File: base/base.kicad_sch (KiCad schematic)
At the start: 1 part, among them U1 ESP32-WROOM-32

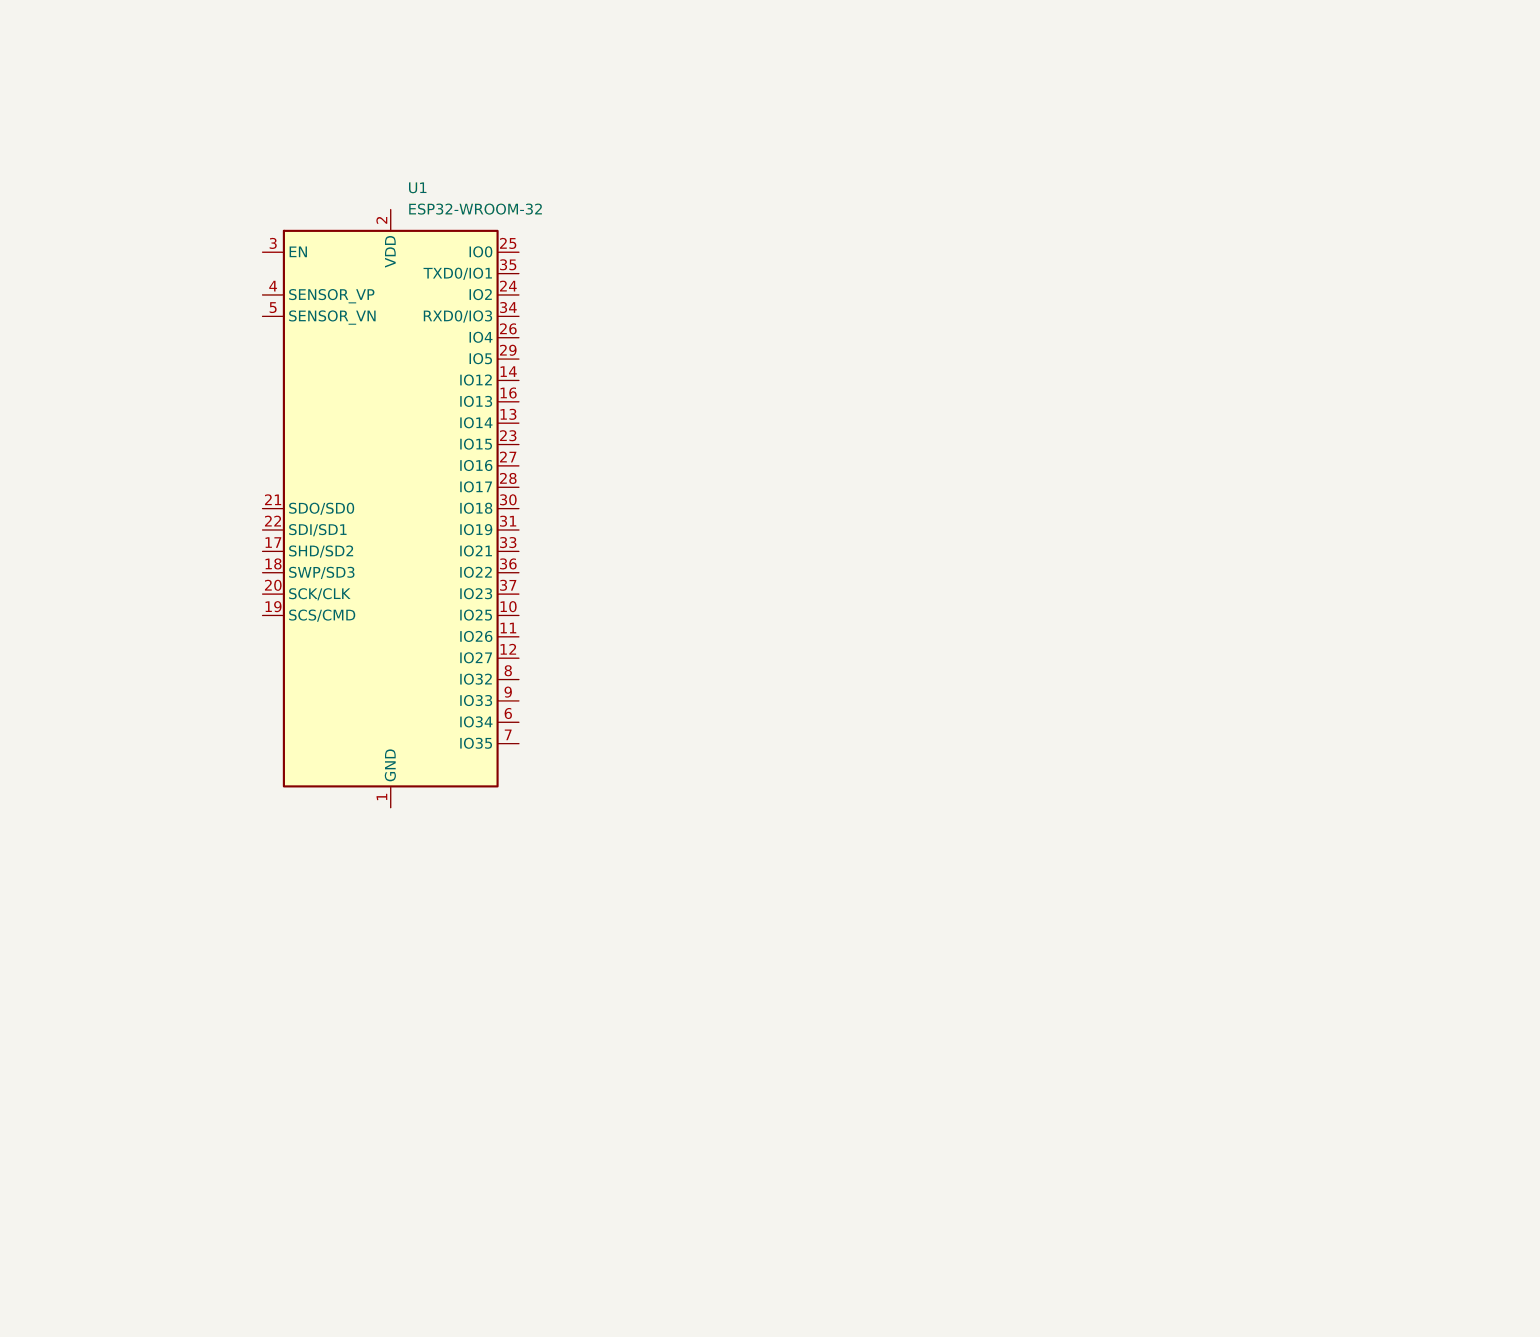
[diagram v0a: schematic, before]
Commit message: add base pcb
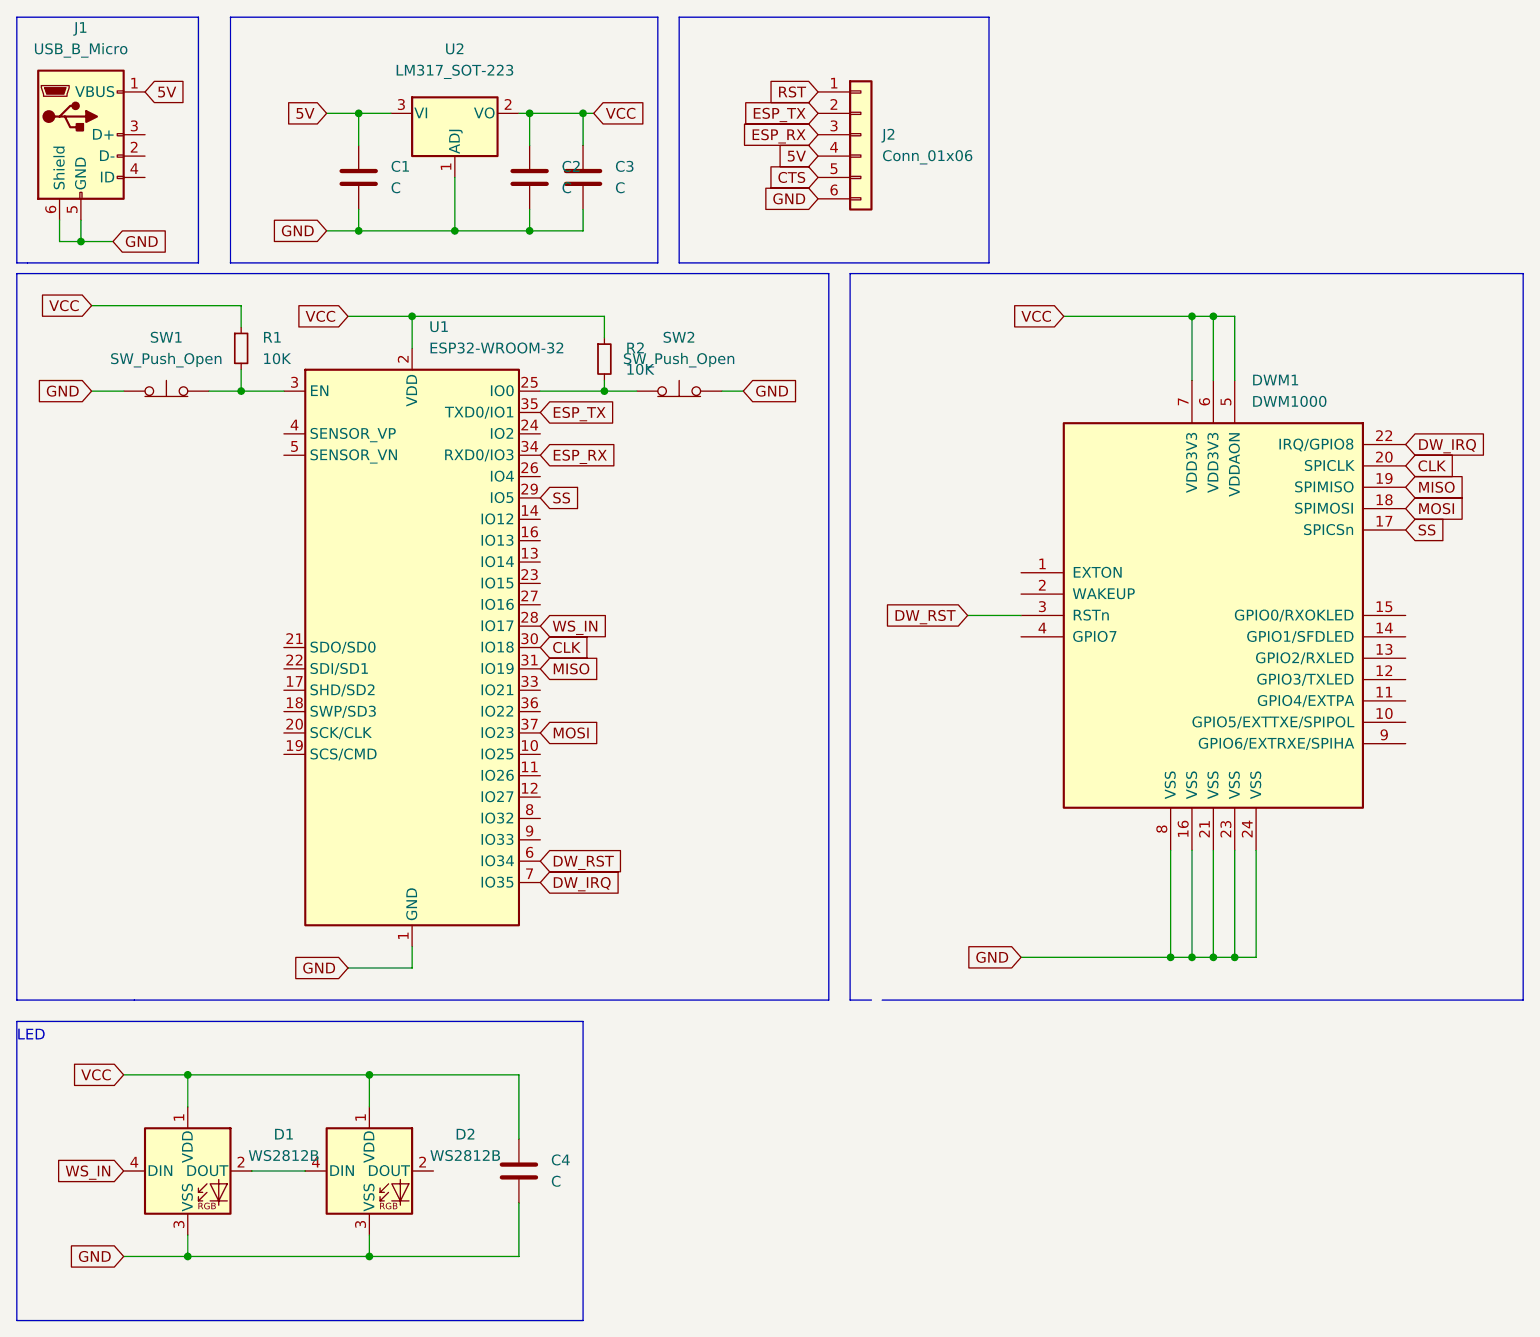
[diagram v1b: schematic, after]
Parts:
- added C1, C2, C3, C4: C, Capacitor_SMD:C_0603_1608Metric, symbol Device:C
- added D1, D2: WS2812B, LED_SMD:LED_WS2812B_PLCC4_5.0x5.0mm_P3.2mm, symbol LED:WS2812B
- added DWM1: DWM1000, RF_Module:DWM1000, symbol RF_Module:DWM1000
- added J1: USB_B_Micro, Connector_USB:USB_Micro-B_Molex-105017-0001, symbol Connector:USB_B_Micro
- added J2: Conn_01x06, Connector_PinHeader_2.54mm:PinHeader_1x06_P2.54mm_Vertical, symbol Connector_Generic:Conn_01x06
- added R1, R2: 10K, Resistor_SMD:R_0603_1608Metric, symbol Device:R_Small
- added SW1, SW2: SW_Push_Open, Button_Switch_SMD:SW_SPST_CK_RS282G05A3, symbol Switch:SW_Push_Open
- added U2: LM317_SOT-223, Package_TO_SOT_SMD:SOT-223-3_TabPin2, symbol Regulator_Linear:LM317_SOT-223
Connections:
- net GND: now reaches U1.1 (GND), U1.15 (GND), U1.38 (GND), U1.39 (GND)
- net GND: now also C1.2, C2.2, C3.2, C4.2, D1.3 (VSS), D2.3 (VSS), DWM1.16 (VSS), DWM1.21 (VSS), DWM1.23 (VSS), DWM1.24 (VSS), DWM1.8 (VSS), J1.5 (GND), J1.6 (Shield), J2.6 (Pin_6), SW1.1 (A), SW2.2 (B), U2.1 (ADJ)
- net VCC: now reaches U1.2 (VDD)
- net VCC: now also C2.1, C3.1, C4.1, D1.1 (VDD), D2.1 (VDD), DWM1.5 (VDDAON), DWM1.6 (VDD3V3), DWM1.7 (VDD3V3), R1.1, R2.1, U2.2 (VO)
- net at U1.25 (IO0): now also R2.2, SW2.1 (A)
- net WS_IN: now reaches U1.28 (IO17)
- net WS_IN: now also D1.4 (DIN)
- net SS: now reaches U1.29 (IO5)
- net SS: now also DWM1.17 (SPICSn)
- net at U1.3 (EN): now also R1.2, SW1.2 (B)
- net CLK: now reaches U1.30 (IO18)
- net CLK: now also DWM1.20 (SPICLK)
- net MISO: now reaches U1.31 (IO19)
- net MISO: now also DWM1.19 (SPIMISO)
- net ESP_RX: now reaches U1.34 (RXD0/IO3)
- net ESP_RX: now also J2.3 (Pin_3)
- net ESP_TX: now reaches U1.35 (TXD0/IO1)
- net ESP_TX: now also J2.2 (Pin_2)
- net MOSI: now reaches U1.37 (IO23)
- net MOSI: now also DWM1.18 (SPIMOSI)
- net DW_RST: now reaches U1.6 (IO34)
- net DW_RST: now also DWM1.3 (RSTn)
- net DW_IRQ: now reaches U1.7 (IO35)
- net DW_IRQ: now also DWM1.22 (IRQ/GPIO8)
- new net: D1.2 (DOUT), D2.4 (DIN)
- new net 5V: C1.1, J1.1 (VBUS), J2.4 (Pin_4), U2.3 (VI)
- new net CTS: J2.5 (Pin_5)
- new net RST: J2.1 (Pin_1)
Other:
- note added: "LED"
- moved on the sheet: U1
